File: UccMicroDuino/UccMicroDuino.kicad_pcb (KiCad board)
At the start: 2 copper layers, 45 x 45 mm, 14 parts, among them J1 Pcb USB Type A, J2 Header, U1 ATtiny85-20SU

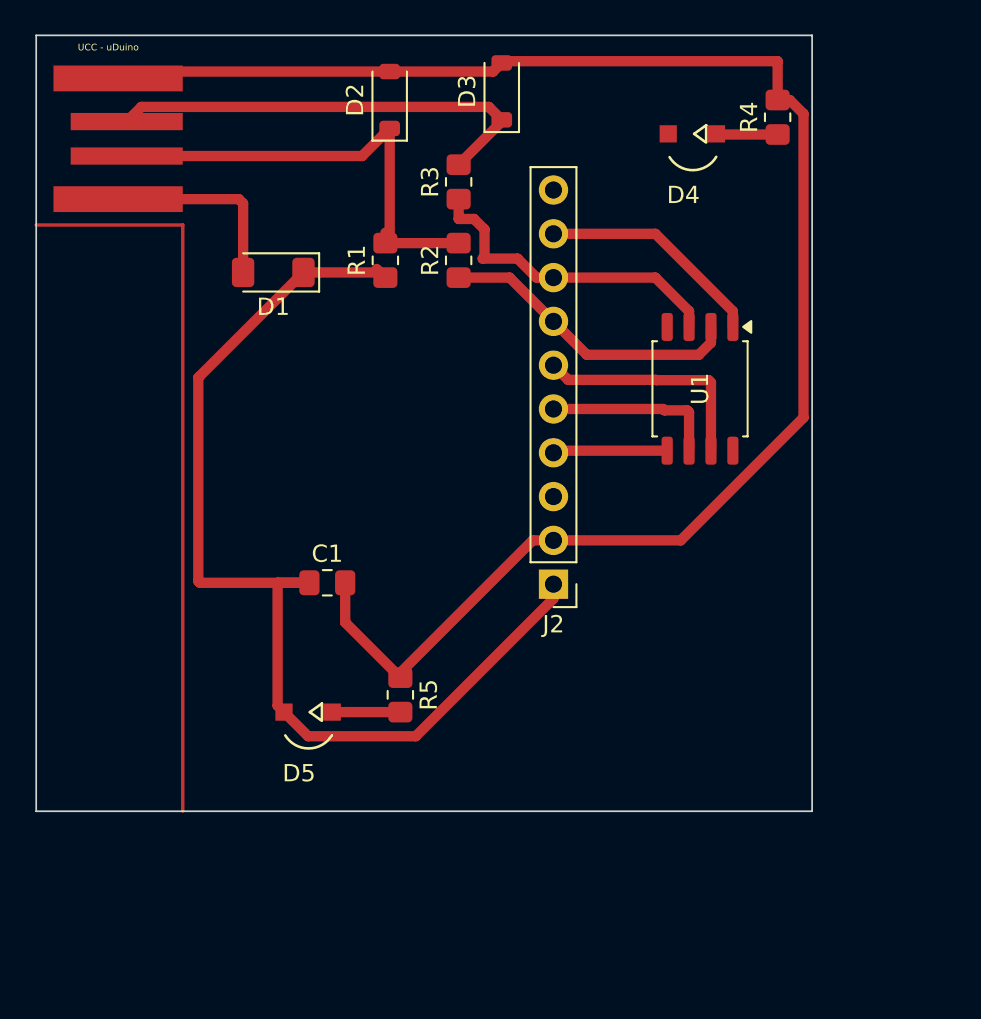
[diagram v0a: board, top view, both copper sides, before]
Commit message: Add files via upload
Actualización proyecto KiCad
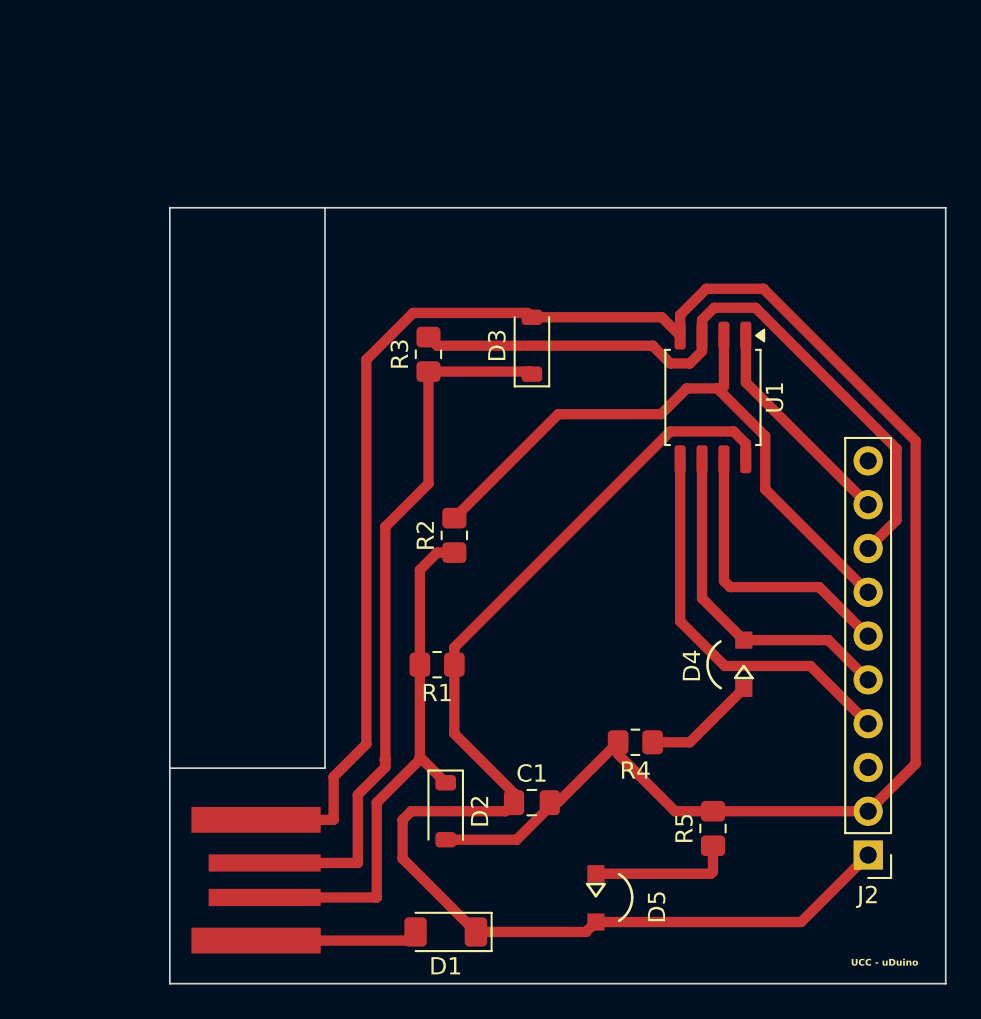
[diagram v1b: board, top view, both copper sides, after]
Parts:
- D3: value 3.6v 1/2mW -> 3.6V 1/2mW
- D4: value Led Green -> LED Green
- D5: value Led Red -> LED Red
- R1: value 1.5KΩ 5% 1/8W -> 1.5KΩ 5% 1/8w
- R2, R3: value 68Ω 5% 1/8W -> 68Ω 5% 1/8W
- moved J1 43.7 mm to (177.2, 110.0)
- moved D2 41.4 mm to (188.0, 106.0), turned to -90 degrees
- moved D1 39.5 mm to (188.0, 113.0)
- moved R4 37.2 mm to (199.0, 102.0), turned to 180 degrees
- moved D4 30.6 mm to (205.3, 97.1), turned to 90 degrees
- moved J2 24.1 mm to (212.5, 108.5)
- moved R1 23.6 mm to (187.5, 97.5), turned to 180 degrees
- moved D5 20.4 mm to (196.7, 111.4), turned to -90 degrees
- moved R5 19.7 mm to (203.5, 107.0), turned to 90 degrees
- moved C1 17.4 mm to (193.0, 105.5)
- moved R2 16.0 mm to (188.5, 90.0)
- moved D3 14.9 mm to (193.0, 79.0)
- moved R3 10.2 mm to (187.0, 79.5)
- moved U1 0.90 mm to (203.5, 82.0)
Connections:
- R2 pad 1: Net-(J2-Pin_7) -> Net-(D2-K)
- R2 pad 2: Net-(D2-K) -> Net-(J2-Pin_7)
- R3 pad 1: Net-(J2-Pin_8) -> Net-(D3-K)
- R3 pad 2: Net-(D3-K) -> Net-(J2-Pin_8)
- R5 pad 1: GND -> Net-(D5-K)
- R5 pad 2: Net-(D5-K) -> GND
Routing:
- net GND: track 97.0 -> 122.6 mm
- net Net-(J2-Pin_8): track 18.8 -> 40.0 mm
- net Net-(J2-Pin_7): track 17.7 -> 37.1 mm
- net Net-(J2-Pin_4): track 6.65 -> 22.8 mm
- net Net-(D3-K): track 26.2 -> 41.7 mm
- net +5V: track 62.3 -> 73.5 mm
- net Net-(D4-A): track 10.2 -> 19.7 mm
- net Net-(D5-K): track 3.95 -> 8.34 mm
- net Net-(D2-K): track 27.5 -> 31.1 mm
- net Net-(J2-Pin_6): track 13.5 -> 16.7 mm
- net Net-(D4-K): track 3.56 -> 6.58 mm
- net Net-(D1-A): track 11.4 -> 9.46 mm
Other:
- outline, holes or cut-outs redrawn
